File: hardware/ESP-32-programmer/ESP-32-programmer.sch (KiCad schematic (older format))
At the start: 18 parts, among them J1 GS2, J2 CONN_01X06, J3 CONN_02X10, J4 CONN_02X10, J5 CONN_02X10, J6 CONN_01X06, J7 GS2, J8 GS2, SW1 SW_DIP_x02, SW2 SW_Push, U1 LD1117S33TR_SOT223, U2 ESP-32-module

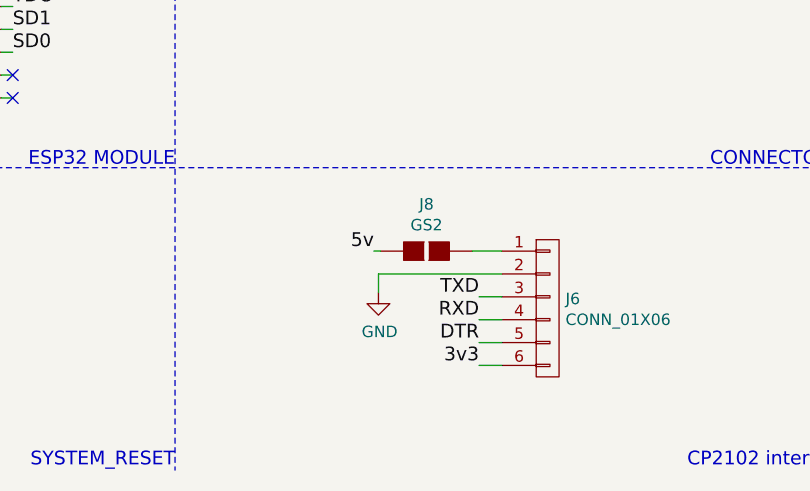
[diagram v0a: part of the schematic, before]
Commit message: Move solder bridge on CP2012 programmer header
1. Move the solder bridge on the CP2012 header from 5v line to 3.3v line to prevent voltage fed to LDO(5v) output(3v3) from feeding back to the CP2102 3v3 output. This would allow unwanted currents to flow between the supplies.
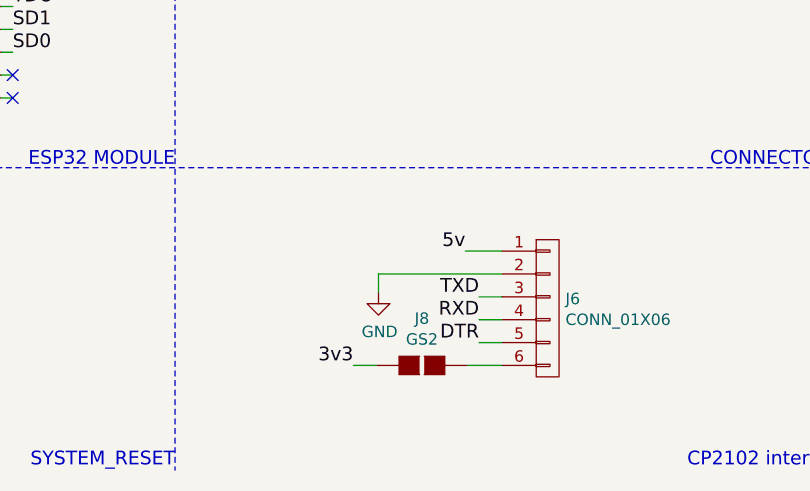
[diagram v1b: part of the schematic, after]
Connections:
- net 3v3: now also J8.2 (G2); no longer J6.6 (P6)
- net 5v: now also J6.1 (P1); no longer J8.2 (G2)
- net at J8.1 (G1): now also J6.6 (P6); no longer J6.1 (P1)
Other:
- moved on the sheet: J8
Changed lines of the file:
@@
 	1    0    0    -1
 $EndComp
-Text Label 9140 5580 2    60   ~ 0
+Text Label 9540 5580 2    60   ~ 0
 5v
 Text Label 9600 5780 2    60   ~ 0
@@
 Text Label 9600 5880 2    60   ~ 0
 RXD
-Text Label 9600 6080 2    60   ~ 0
-3v3
 $Comp
 L GS2 J1
@@
 	8270 5220 8270 6540
 Wire Wire Line
-	9570 5580 9700 5580
+	9540 5580 9700 5580
 Wire Wire Line
 	9160 5680 9700 5680
@@
 	9160 5760 9160 5680
 Wire Wire Line
-	9700 6080 9600 6080
+	9550 6080 9700 6080
 Wire Wire Line
 	1850 1250 1590 1250
@@
 L GS2 J8
 U 1 1 59A5D683
-P 9370 5580
-F 0 "J8" V 9165 5580 50  0000 C CNN
-F 1 "GS2" V 9256 5580 50  0000 C CNN
-F 2 "Connectors:GS2" V 9444 5580 50  0001 C CNN
-F 3 "" H 9370 5580 50  0001 C CNN
-	1    9370 5580
+P 9350 6080
+F 0 "J8" V 9145 6080 50  0000 C CNN
+F 1 "GS2" V 9236 6080 50  0000 C CNN
+F 2 "Connectors:GS2" V 9424 6080 50  0001 C CNN
+F 3 "" H 9350 6080 50  0001 C CNN
+	1    9350 6080
 	0    1    1    0
 $EndComp
-Wire Wire Line
-	9140 5580 9170 5580
 Text Label 7560 3310 0    60   ~ 0
 RXD
+Wire Wire Line
+	9150 6080 9050 6080
+Text Label 9050 6080 2    60   ~ 0
+3v3
 $EndSCHEMATC
